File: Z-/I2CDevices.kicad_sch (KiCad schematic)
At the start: 40 parts, among them U1 OPT4003DNPRQ1, U2 LTC4316xDD, U3 ADM1176-1ARMZ-R7, U4 NCV891330PD50R2G, U5 DRV8830DRC

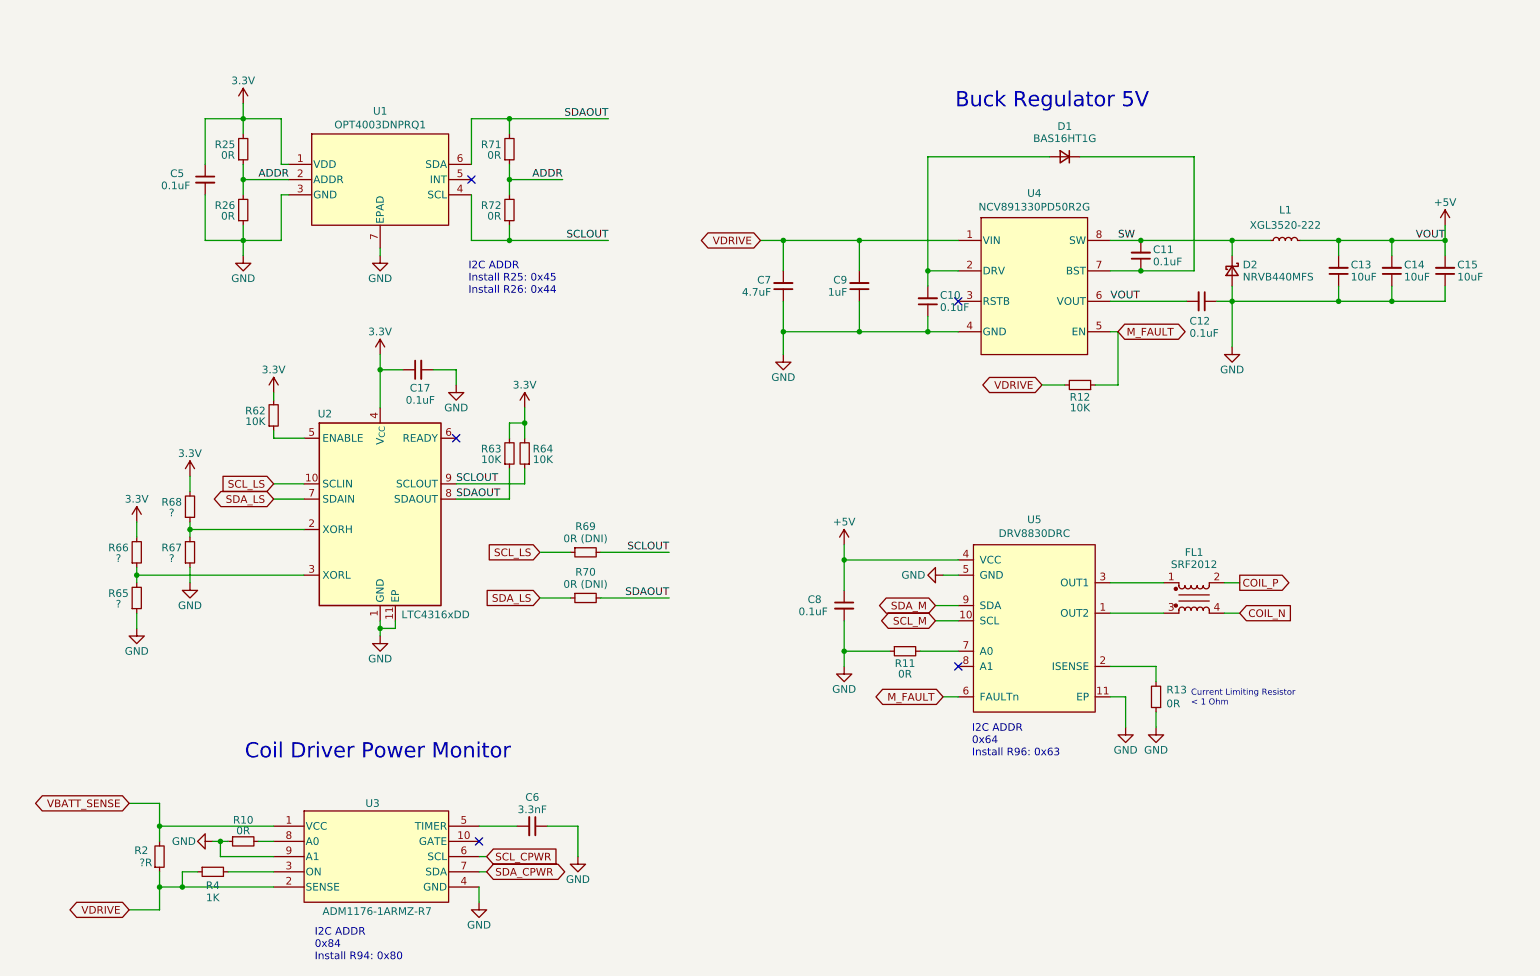
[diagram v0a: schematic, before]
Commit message: Z- Solar Panel files upload
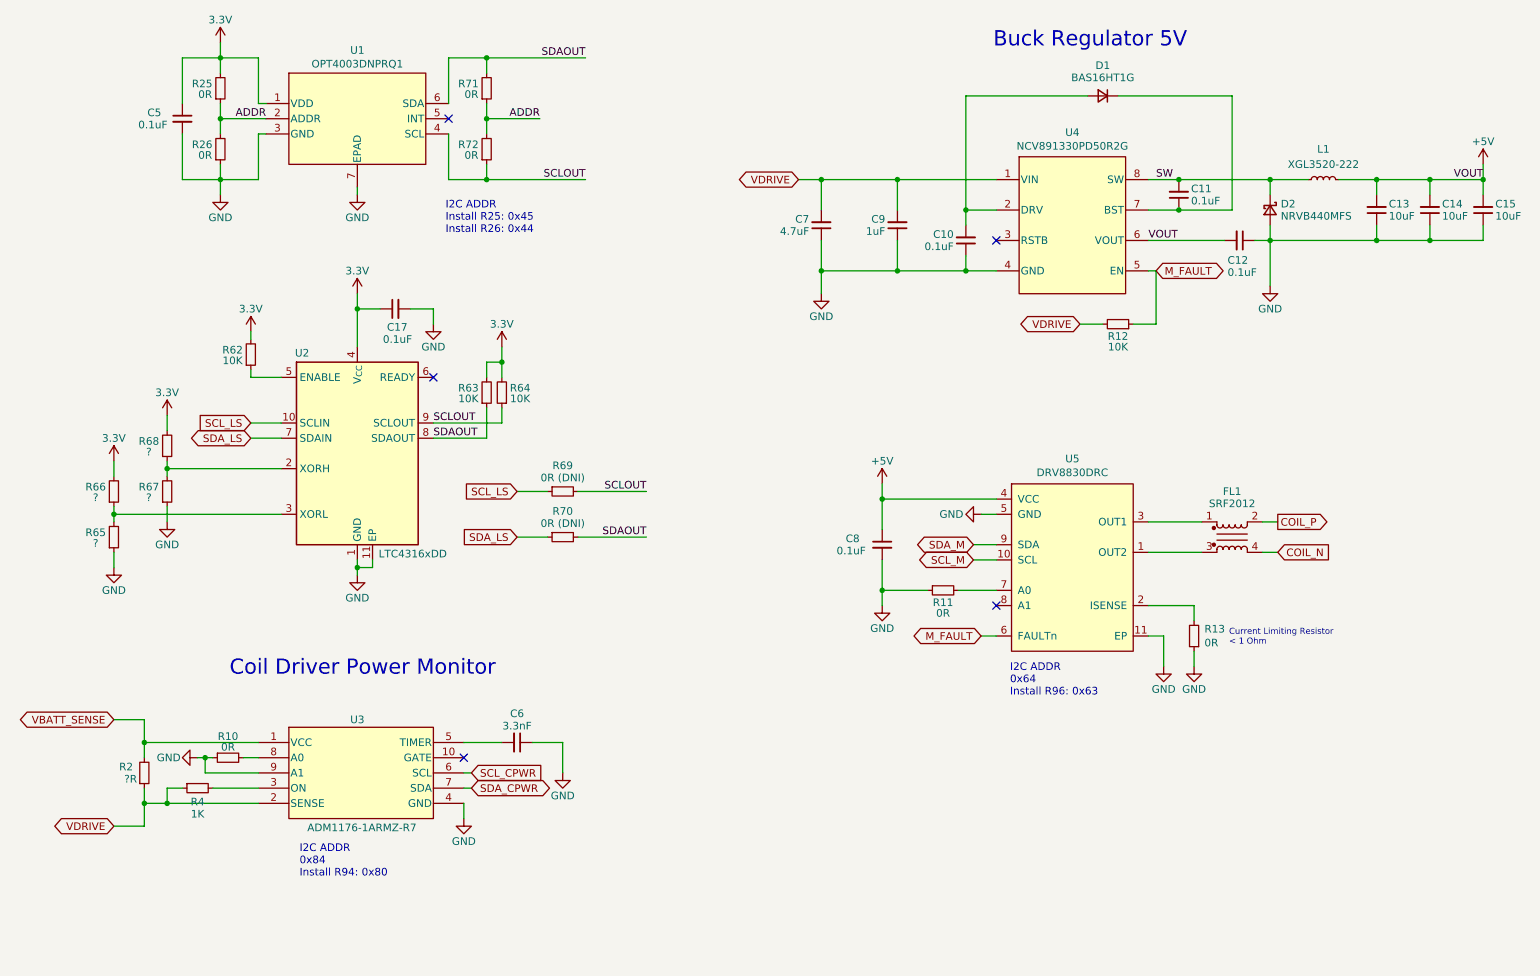
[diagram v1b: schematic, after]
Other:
- moved on the sheet: C10, C11, C12, C13, C14, C15, C17, C5, C6, C7, C8, C9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
